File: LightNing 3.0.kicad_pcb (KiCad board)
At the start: 2 copper layers, 55 x 48 mm, 32 parts, among them J1 motores izq, J2 motores der, J4 esp32 usb y batt, J6 batt, J8 LED_izq, J9 LED_izq, SW1 SW_SPDT, U1 L298(H)N, U3 L7805, U4 ESP32-WROOM-E, U5 AMS1117-3.3

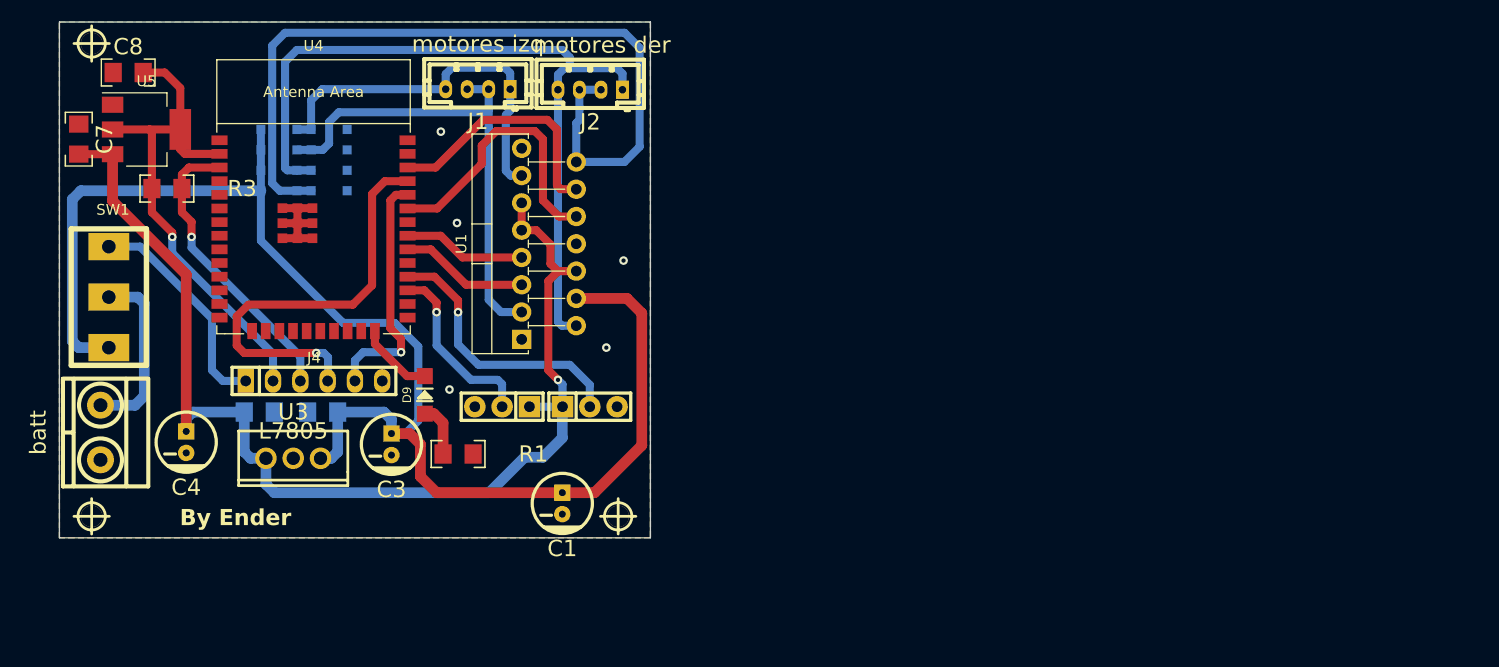
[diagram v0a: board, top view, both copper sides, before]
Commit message: pcb terminado
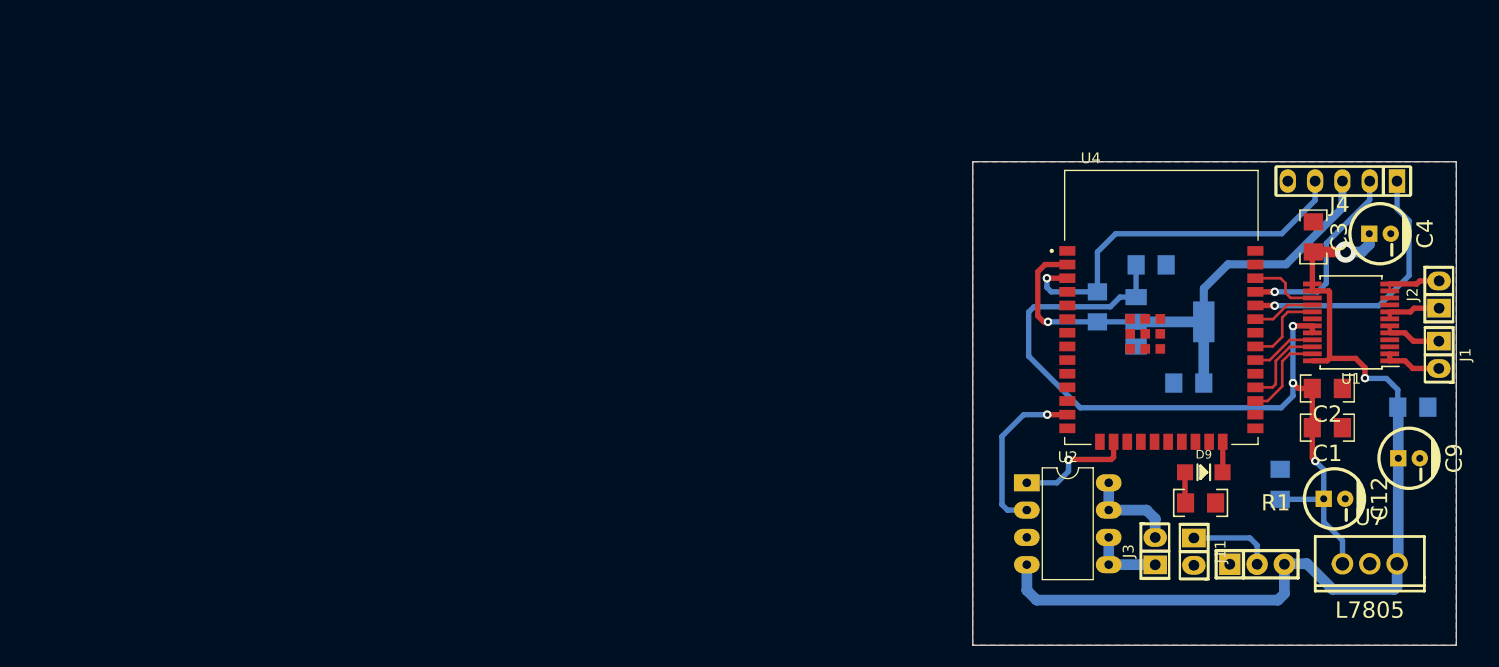
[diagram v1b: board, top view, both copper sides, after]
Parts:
- removed C5, C6: 100nF, EESTN5:C_1206
- removed D1, D2, D3, D4, D5, D6, D7, D8: 1n4001, EESTN5:sod123
- removed J6: batt, EESTN5:BORNERA2_AZUL
- removed J8, J9: LED_izq, EESTN5:Pin_Strip_3
- removed R3: 10k, EESTN5:R_1206
- removed SW1: SW_SPDT, EESTN5:SW_SPDT_TH_Vertical
- removed U3: L7805, EESTN5:TO-220
- removed hole_2mm (x3): VAL**, EESTN5:hole_2mm
- added C10: 100nF, EESTN5:C_1206, B.Cu at (165.9, 57.8)
- added C11: 100nF, EESTN5:C_1206, B.Cu at (153.6, 65.0)
- added C12: 10uF 16v, EESTN5:CAP_ELEC_5x11mm, F.Cu at (158.7, 66.4)
- added C2: 100nF, EESTN5:C_1206, F.Cu at (158.0, 56.1)
- added C9: 100uF 25v, EESTN5:CAP_ELEC_5x11mm, F.Cu at (165.6, 62.6)
- added J11: batt, EESTN5:Pin_Header_2, F.Cu at (145.9, 71.3)
- added J3: motor dir, EESTN5:Pin_Header_2, F.Cu at (141.7, 71.2)
- added R2: 10k, EESTN5:R_1206, B.Cu at (136.6, 48.5)
- added SW2: SW_SPDT, EESTN5:Pin_Strip_3, F.Cu at (151.5, 72.5)
- added U2: TA6586, EESTN5:DIP-8, F.Cu at (130.0, 64.9)
- added U7: L7805, EESTN5:TO-220, F.Cu at (161.9, 72.4)
- C1: value 220uf -> 10uF; footprint EESTN5:CAP_ELEC_5x11mm -> EESTN5:C_1206
- C3: value 100uF 25v -> 10uF; footprint EESTN5:CAP_ELEC_5x11mm -> EESTN5:C_1206
- C4: value 10uF 16v -> 22uF 25v
- C7, C8, U5: moved to B.Cu
- J1: value motores izq -> motor izq; footprint EESTN5:JST-4V -> EESTN5:Pin_Header_2
- J2: value motores der -> motor der; footprint EESTN5:JST-4V -> EESTN5:Pin_Header_2
- J4: value esp32 usb y batt -> programmer; footprint EESTN5:Pin_Header_6 -> EESTN5:Pin_Strip_5
- U1: value L298(H)N -> TB6612FNG; footprint Package_TO_SOT_THT:TO-220-15_P2.54x2.54mm_StaggerEven_Lead4.58mm_Vertical -> Package_SO:SSOP-24_5.3x8.2mm_P0.65mm
- U4: footprint Espressif:ESP32-WROOM-32E -> esp32e:XCVR_ESP32-WROOM-32E__16MB_
- moved C4 112.8 mm to (162.9, 41.7), turned to -90 degrees
- moved C8 102.8 mm to (145.1, 55.6)
- moved C7 100.5 mm to (141.6, 44.6), turned to 180 degrees
- moved J4 97.5 mm to (159.4, 36.8), turned to 180 degrees
- moved U5 96.9 mm to (143.3, 49.9)
- moved J1 93.1 mm to (168.7, 53.0), turned to -90 degrees
- moved C3 87.9 mm to (156.7, 42.0), turned to -90 degrees
- moved J2 81.0 mm to (168.1, 47.4), turned to 90 degrees
- moved U4 79.4 mm to (142.6, 48.6)
- moved U1 77.2 mm to (160.2, 50.0), turned to 180 degrees
- moved D9 72.9 mm to (146.5, 63.9), turned to 0 degrees
- moved C1 71.5 mm to (158.0, 59.8)
- moved R1 69.2 mm to (146.2, 66.8)
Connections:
- C1 pad 1: VCC -> +5V
- C4 pad 1: +5V -> VCC
- J1 pad 1: Net-(D7-A) -> Net-(J1-Pad1)
- J1 pad 2: Net-(D1-A) -> Net-(J1-Pad2)
- J2 pad 1: Net-(D3-A) -> Net-(J2-Pad1)
- J2 pad 2: Net-(D5-A) -> Net-(J2-Pad2)
- J4 pad 1: /salida -> /rx
- J4 pad 2: +3.3V -> /tx
- J4 pad 3: /EN -> +3.3V
- J4 pad 4: /TX -> /en
- J4 pad 5: /RX -> GND
- U1 pad 1: GND -> Net-(J1-Pad2)
- U1 pad 10: /IN4 -> GND
- U1 pad 11: +5V -> Net-(J2-Pad2)
- U1 pad 12: /IN3 -> Net-(J2-Pad2)
- U1 pad 13: Net-(D7-A) -> VCC
- U1 pad 14: Net-(D5-A) -> VCC
- U1 pad 15: GND -> /PWB
- U1 pad 2: Net-(D3-A) -> Net-(J1-Pad2)
- U1 pad 3: Net-(D1-A) -> GND
- U1 pad 4: VCC -> GND
- U1 pad 5: /IN2 -> Net-(J1-Pad1)
- U1 pad 6: +5V -> Net-(J1-Pad1)
- U1 pad 7: /IN1 -> Net-(J2-Pad1)
- U1 pad 8: GND -> Net-(J2-Pad1)
- U1 pad 9: +5V -> GND
- U4 pad 10: unconnected-(U4-DAC_1/ADC2_CH8/GPIO25-Pad10) -> /buzz
- U4 pad 13: unconnected-(U4-MTMS/GPIO14/ADC2_CH6-Pad13) -> /pin_dirA
- U4 pad 16: unconnected-(U4-MTCK/GPIO13/ADC2_CH4-Pad16) -> /pin_dirB
- U4 pad 27: /Led_Izq -> /PWA
- U4 pad 28: /Led_Der -> /IN2
- U4 pad 3: /EN -> /en
- U4 pad 30: /IN2 -> /IN1
- U4 pad 31: /IN1 -> /IN3
- U4 pad 34: /RX -> /rx
- U4 pad 35: /TX -> /tx
- U4 pad 36: /IN3 -> /PWB
- U4 pad 9: unconnected-(U4-32K_XN/GPIO33/ADC1_CH5-Pad9) -> /led
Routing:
- net Net-(D5-A): track 76.5 -> 0.00 mm
- net Net-(D3-A): track 73.5 -> 0.00 mm
- net VCC: track 134.0 -> 87.6 mm, vias 0 -> 2
- net Net-(D1-A): track 45.7 -> 0.00 mm
- net /TX: track 40.1 -> 0.00 mm, vias 1 -> 0
- net Net-(D7-A): track 35.8 -> 0.00 mm
- net /en: track 0.00 -> 35.4 mm, vias 0 -> 1
- net +5V: track 108.5 -> 77.6 mm, vias 1 -> 3
- net /EN: track 27.5 -> 0.00 mm, vias 1 -> 0
- net /Led_Der: track 25.6 -> 0.00 mm, vias 1 -> 0
- net /rx: track 0.00 -> 25.1 mm, vias 0 -> 1
- net /RX: track 22.9 -> 0.00 mm, vias 1 -> 0
- net /salida: track 20.7 -> 0.00 mm
- net /IN4: track 26.3 -> 5.85 mm
- net /tx: track 0.00 -> 18.4 mm, vias 0 -> 1
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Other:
- board size 55 x 48 mm -> 45 x 45 mm
- board text removed: "By Ender"
